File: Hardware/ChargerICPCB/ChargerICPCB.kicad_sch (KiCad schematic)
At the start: 18 parts, among them J1 SLIMSTACK, J2 CarLVPowerConnector, U1 LTC4011CFE

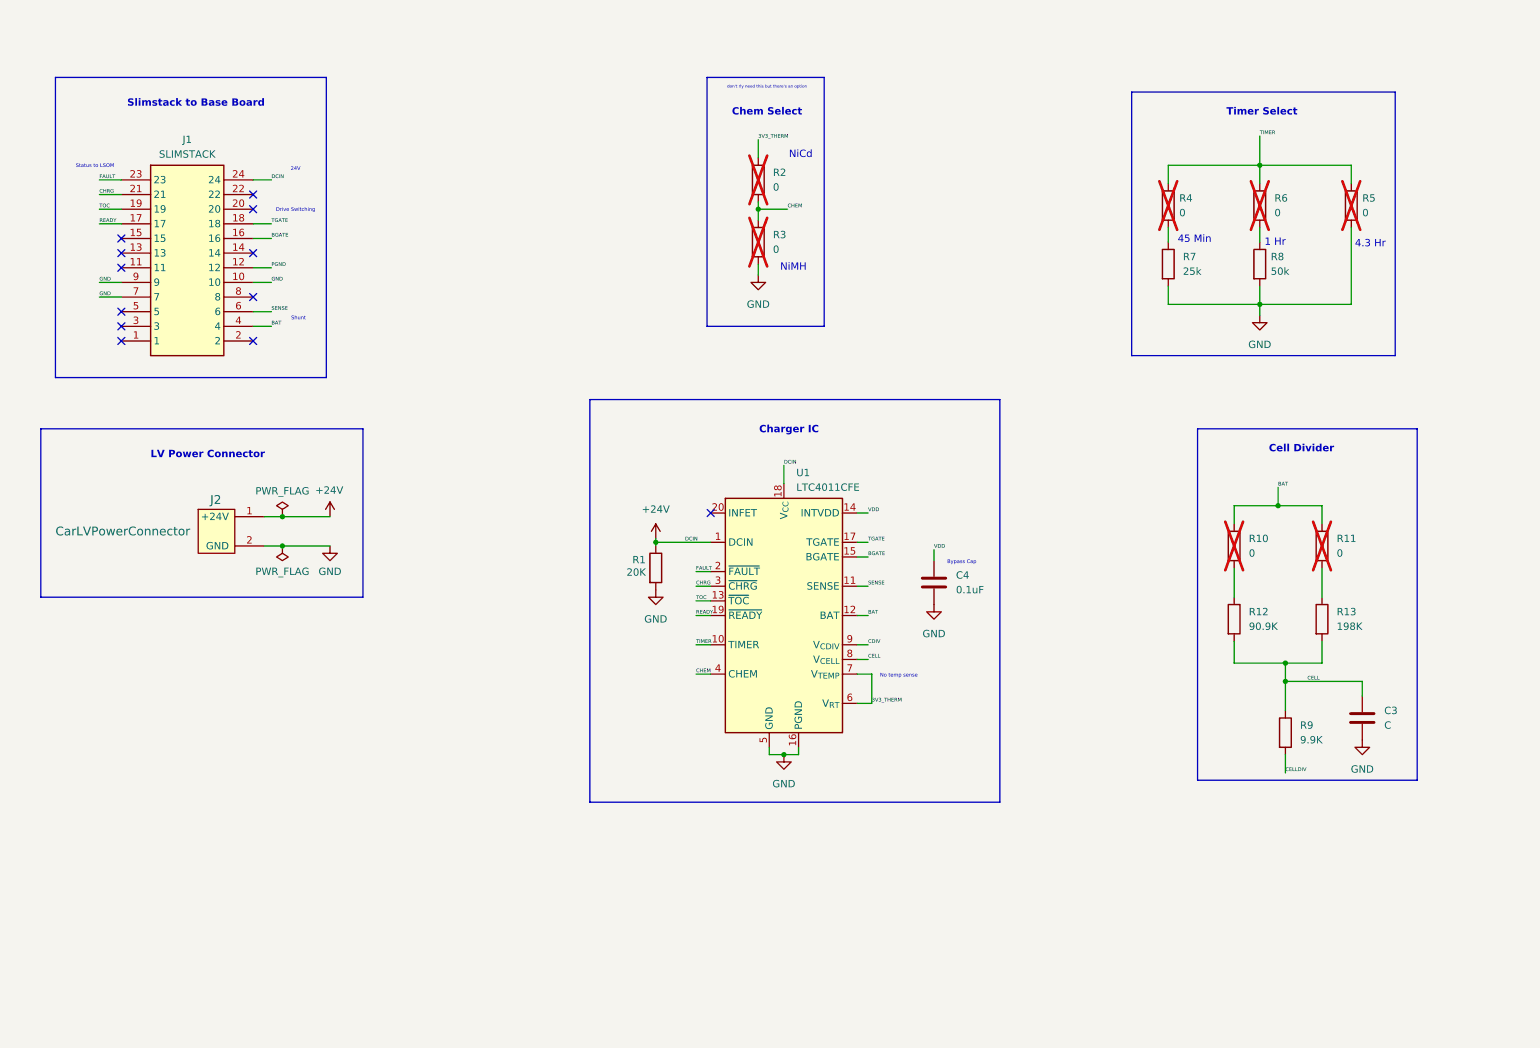
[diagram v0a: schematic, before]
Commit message: schem good
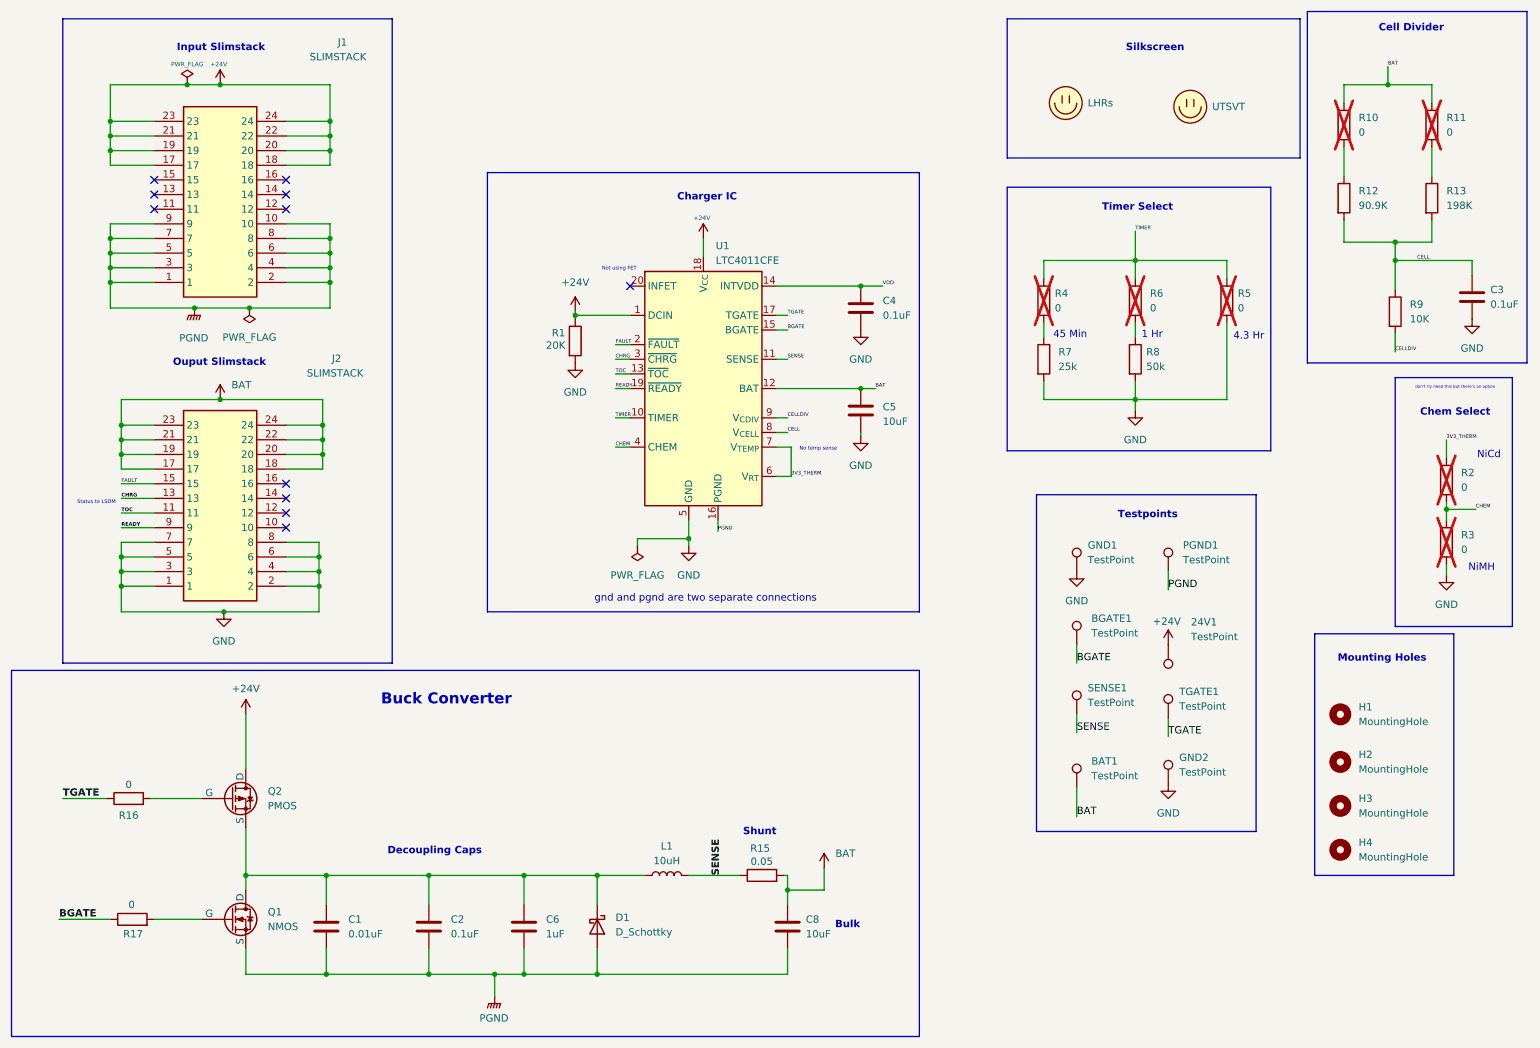
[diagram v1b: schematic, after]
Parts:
- removed J2: CarLVPowerConnector, symbol utsvt_connectors:CarLVPowerConnector
- added 24V1, BAT1, BGATE1, GND1, GND2, PGND1, SENSE1, TGATE1: TestPoint, Connector_PinHeader_1.00mm:PinHeader_1x01_P1.00mm_Vertical, symbol Connector:TestPoint
- added C1: 0.01uF, Capacitor_SMD:C_0201_0603Metric, symbol Device:C
- added C2: 0.1uF, Capacitor_SMD:C_0201_0603Metric, symbol Device:C
- added C5, C8: 10uF, Capacitor_SMD:C_0201_0603Metric, symbol Device:C
- added C6: 1uF, Capacitor_SMD:C_0201_0603Metric, symbol Device:C
- added D1: D_Schottky, CustomLib:UPS140TR7, symbol Device:D_Schottky
- added H1, H2, H3, H4: MountingHole, MountingHole:MountingHole_3.2mm_M3, symbol Mechanical:MountingHole
- added J2: SLIMSTACK, UTSVT_Connectors:524652470, symbol utsvt_connectors:52465-2470
- added L1: 10uH, CustomLib:WE-LHMI_7050, symbol Device:L
- added LOGO1: LHRs, UTSVT_Logos:LHRs_LOGO, symbol utsvt_misc:Logo_Placeholder
- added LOGO2: UTSVT, UTSVT_Logos:UTSVT_Logo_Symbol, symbol utsvt_misc:Logo_Placeholder
- added Q1: NMOS, CustomLib:TSOP6_MO-193C_VIS, symbol Simulation_SPICE:NMOS
- added Q2: PMOS, CustomLib:TSOT23-6-419BL_OSI, symbol Simulation_SPICE:PMOS
- added R15: 0.05, Resistor_SMD:R_0201_0603Metric, symbol Device:R
- added R16, R17: 0, Resistor_SMD:R_0201_0603Metric, symbol Device:R
- C3: value C -> 0.1uF; footprint (none) -> Capacitor_SMD:C_0201_0603Metric
- C4: footprint (none) -> Capacitor_SMD:C_0201_0603Metric
- R1, R10, R11, R12, R13, R2, R3, R4, R5, R6, R7, R8: footprint (none) -> Resistor_SMD:R_0201_0603Metric
- R9: value 9.9K -> 10K; footprint (none) -> Resistor_SMD:R_0201_0603Metric
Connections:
- net CDIV is gone; now on net CELLDIV: U1.9 (V_{CDIV})
- net +24V: now also J1.17, J1.18, J1.19, J1.20, J1.21, J1.22, J1.23, 24V1.1, Q2.1 (D)
- net BAT: now also BAT1.1, C5.1, C8.1, J2.17, J2.18, J2.19, J2.20, J2.21, J2.22, J2.23, J2.24, R15.2; no longer J1.4
- net BGATE: now also BGATE1.1, R17.1; no longer J1.16
- net CHRG: now also J2.13; no longer J1.21
- net FAULT: now also J2.15; no longer J1.23
- net GND: now also C5.2, GND1.1, GND2.1, J2.1, J2.2, J2.3, J2.4, J2.5, J2.6, J2.7, J2.8; no longer J1.10, J1.7, J1.9, U1.16 (PGND)
- net PGND: now also J1.1, J1.10, J1.2, J1.3, J1.4, J1.5, J1.6, J1.7, J1.8, J1.9, U1.16 (PGND), C1.2, C2.2, C6.2, C8.2, D1.2 (A), PGND1.1, Q1.3 (S); no longer J1.12
- net READY: now also J2.9; no longer J1.17
- net SENSE: now also L1.2, R15.1, SENSE1.1; no longer J1.6
- net TGATE: now also R16.1, TGATE1.1; no longer J1.18
- net TOC: now also J2.11; no longer J1.19
- new net: C1.1, C2.1, C6.1, D1.1 (K), L1.1, Q1.1 (D), Q2.3 (S)
- new net: Q2.2 (G), R16.2
- new net: Q1.2 (G), R17.2
- no-connect marks 12 -> 11
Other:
- note added: "Buck Converter"
- note added: "Bulk"
- note added: "Decoupling Caps"
- note added: "Input Slimstack"
- note added: "Mounting Holes"
- note added: "Not using FET"
- note added: "Ouput Slimstack"
- note added: "Silkscreen"
- note added: "Testpoints"
- note added: "gnd and pgnd are two separate connections"
- note removed: "24V"
- note removed: "Bypass Cap"
- note removed: "Drive Switching"
- note removed: "LV Power Connector"
- note removed: "Slimstack to Base Board"
- moved on the sheet: C3, C4, J1, R1, R10, R11, R12, R13, R2, R3, R4, R5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
